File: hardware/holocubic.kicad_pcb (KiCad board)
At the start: 4 copper layers, 25.5 x 23.5 mm, 48 parts, among them J1 TFT_LCD, J2 USB_C_Receptacle_USB2.0, U1 AMS1117-3.3, U2 ESP32-S3, U3 WM8978, U4 MPU-6050, Y1 40MHz

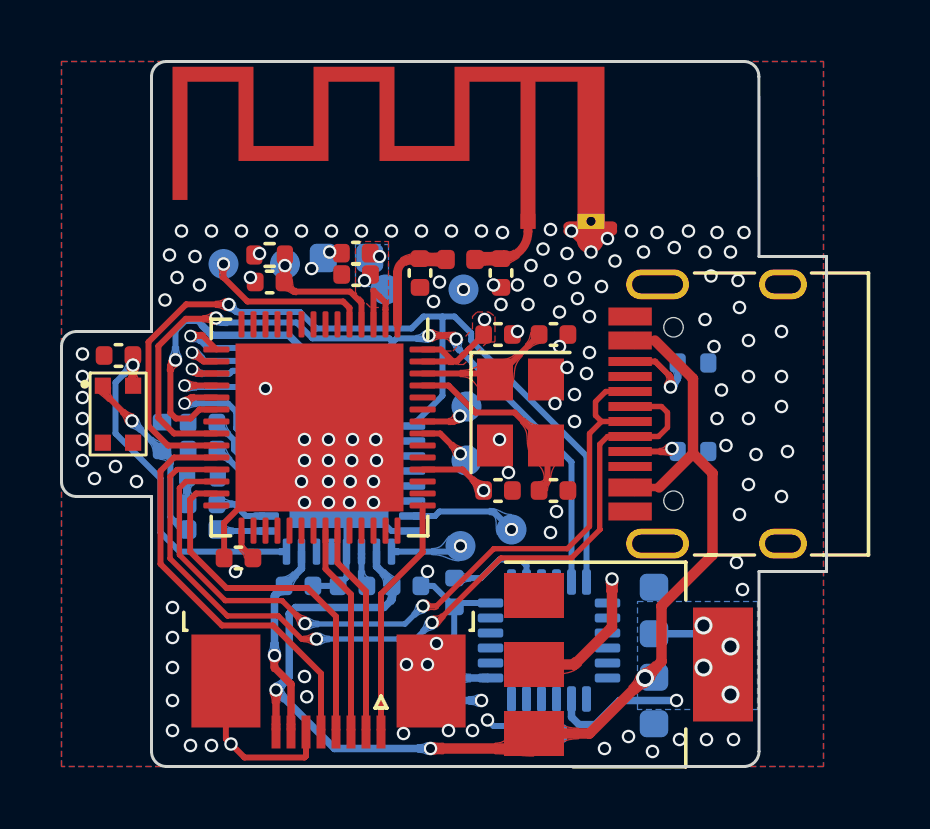
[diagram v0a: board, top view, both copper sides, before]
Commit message: hw: v1.1
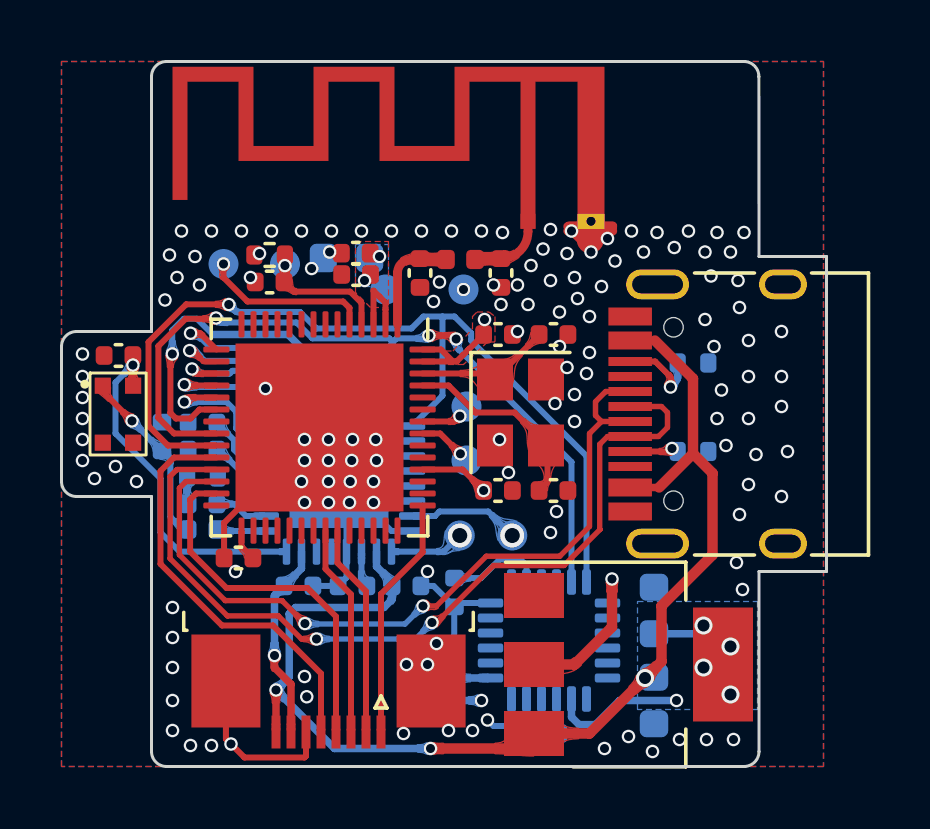
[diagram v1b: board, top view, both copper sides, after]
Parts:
- moved TP7 0.35 mm to (133.3, 112.3)
- moved TP8 0.20 mm to (135.0, 112.3)
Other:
- board text added: "SPK"
